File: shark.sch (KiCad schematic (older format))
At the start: 234 parts, among them J101 USB_B_Mini, Q1 AO4406AL, SW1 MXSwitch, SW10 MXSwitch, SW11 MXSwitch, SW12 MXSwitch, SW13 MXSwitch, SW14 MXSwitch, SW15 MXSwitch, SW16 MXSwitch, SW17 MXSwitch, SW18 MXSwitch, SW19 MXSwitch, SW2 MXSwitch, SW20 MXSwitch, SW21 MXSwitch, SW22 MXSwitch, SW23 MXSwitch, SW24 MXSwitch, SW25 MXSwitch, SW26 MXSwitch, SW27 MXSwitch, SW28 MXSwitch, SW29 MXSwitch, SW3 MXSwitch, SW30 MXSwitch, SW31 MXSwitch, SW32 MXSwitch, SW33 MXSwitch, SW34 MXSwitch, SW35 MXSwitch, SW36 MXSwitch, SW37 MXSwitch, SW38 MXSwitch, SW39 MXSwitch, SW4 MXSwitch, SW40 MXSwitch, SW41 MXSwitch, SW42 MXSwitch, SW43 MXSwitch, SW44 MXSwitch, SW45 MXSwitch, SW46 MXSwitch, SW47 MXSwitch, SW48 MXSwitch, SW49 MXSwitch, SW5 MXSwitch, SW50 MXSwitch, SW51 MXSwitch, SW6 MXSwitch, SW7 MXSwitch, SW8 MXSwitch, SW9 MXSwitch, U1 ATmega32U4-AU, Y1 Crystal

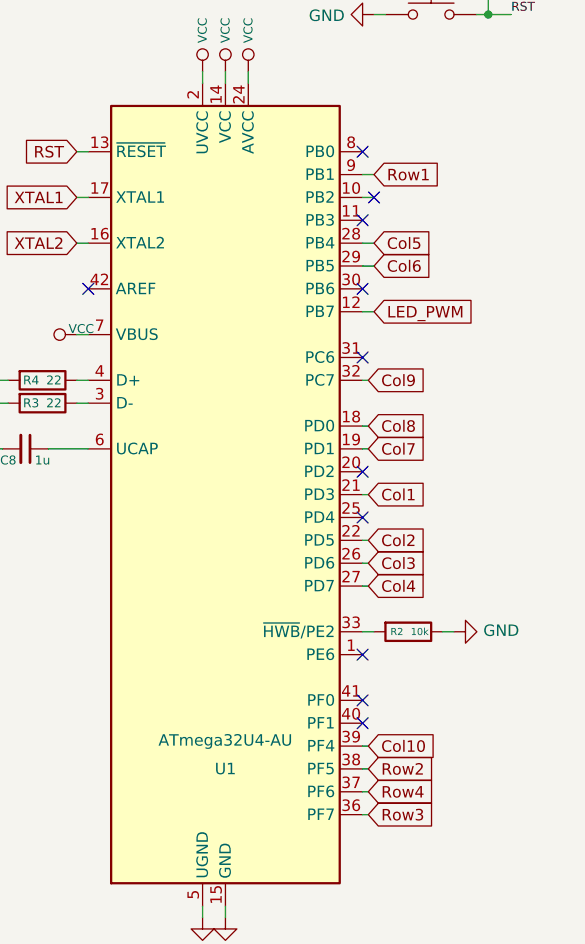
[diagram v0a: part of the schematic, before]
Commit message: Finished routing
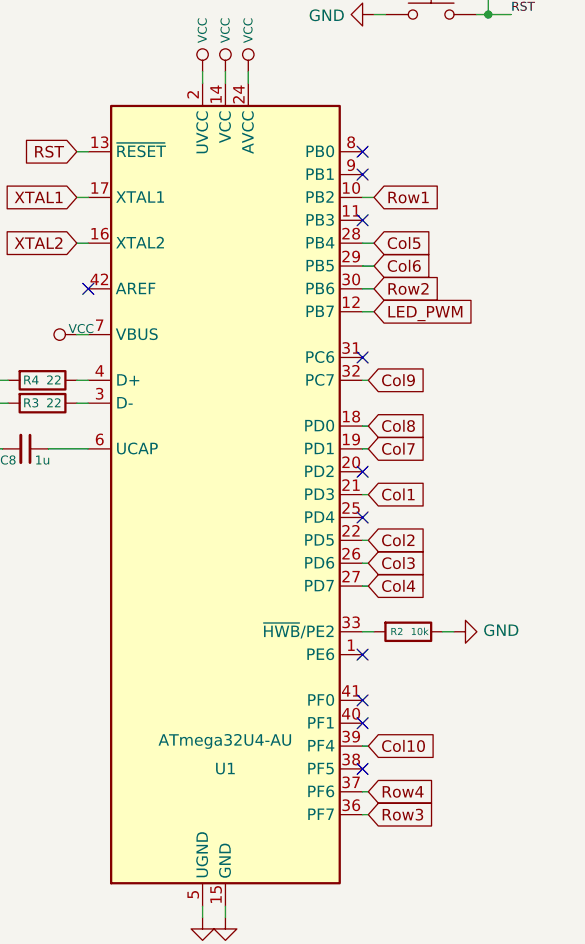
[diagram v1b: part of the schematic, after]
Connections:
- net Row1: now also U1.10 (PB2); no longer U1.9 (PB1)
- net Row2: now also U1.30 (PB6); no longer U1.38 (PF5)
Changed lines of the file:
@@
 Connection ~ 2225 1950
 NoConn ~ 15100 6050
-NoConn ~ 15100 6350
 NoConn ~ 15100 7450
 NoConn ~ 13900 6650
@@
 	14550 4575 14550 4625
 NoConn ~ 15100 8450
-NoConn ~ 15100 6650
 $Comp
 L Device:C_Small C7
@@
 Wire Wire Line
 	15150 6250 15100 6250
-Text GLabel 15150 6150 2    50   Input ~ 0
+Text GLabel 15150 6250 2    50   Input ~ 0
 Row1
-Wire Wire Line
-	15150 6150 15100 6150
 Text GLabel 13500 7050 0    50   Input ~ 0
 D+
@@
 	1    0    0    -1
 $EndComp
-Text GLabel 15125 8750 2    50   Input ~ 0
+Text GLabel 15150 6650 2    50   Input ~ 0
 Row2
-Wire Wire Line
-	15125 8750 15100 8750
-NoConn ~ 15150 6250
 $Comp
 L Keyboard_switches:LED LED49
@@
 $EndComp
 Connection ~ 4200 10150
+NoConn ~ 15100 6150
+NoConn ~ 15100 8750
+Wire Wire Line
+	15150 6650 15100 6650
+NoConn ~ 15100 6350
 $EndSCHEMATC
